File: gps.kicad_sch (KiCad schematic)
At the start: 7 parts, among them J3 50R SMA_Conn, U5 MAX-M10S

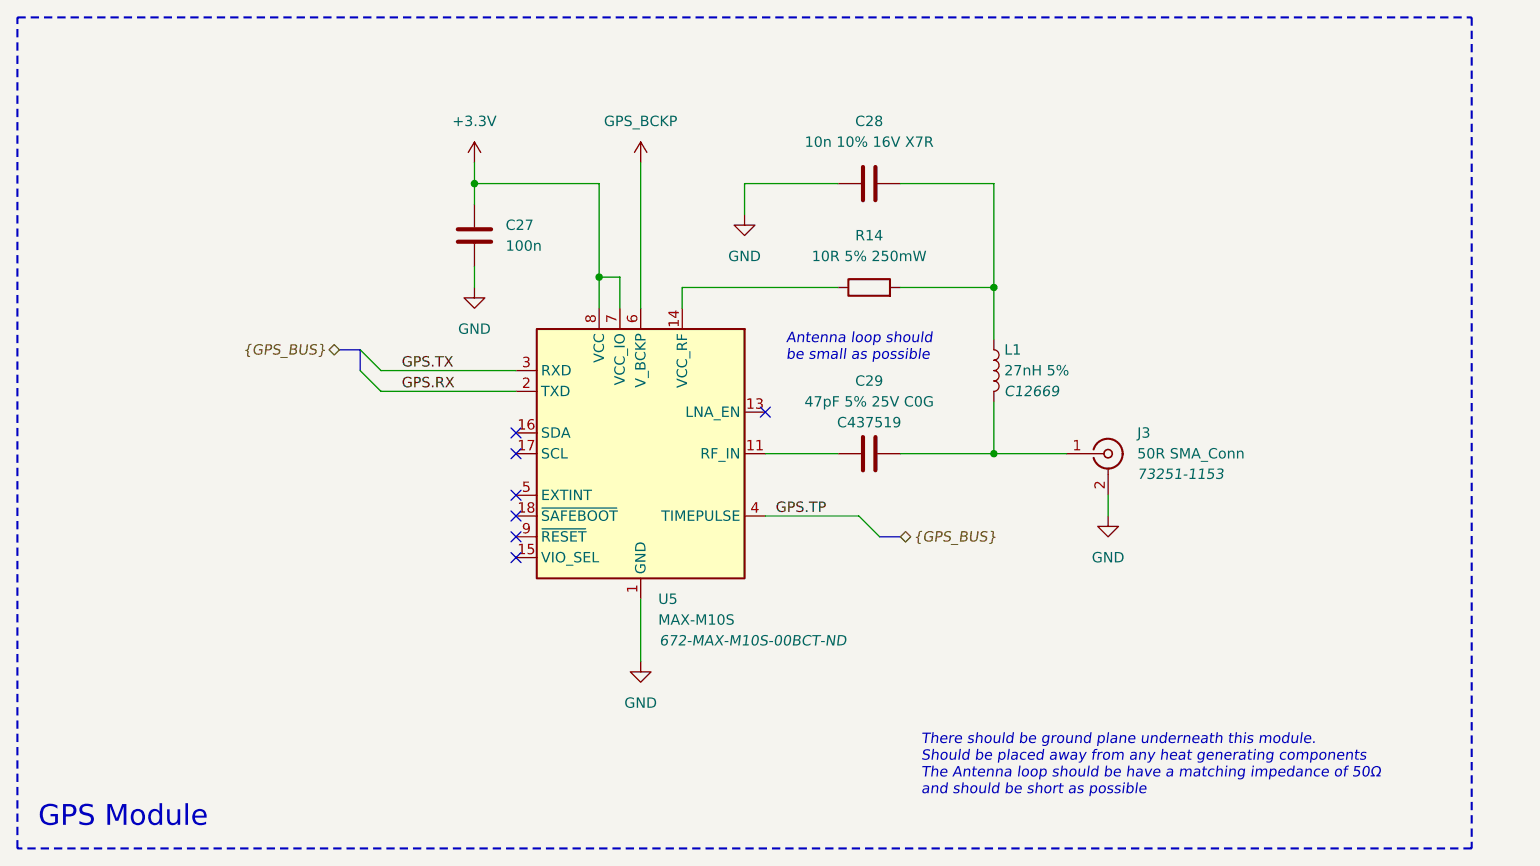
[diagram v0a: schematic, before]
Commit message: PCB Routing
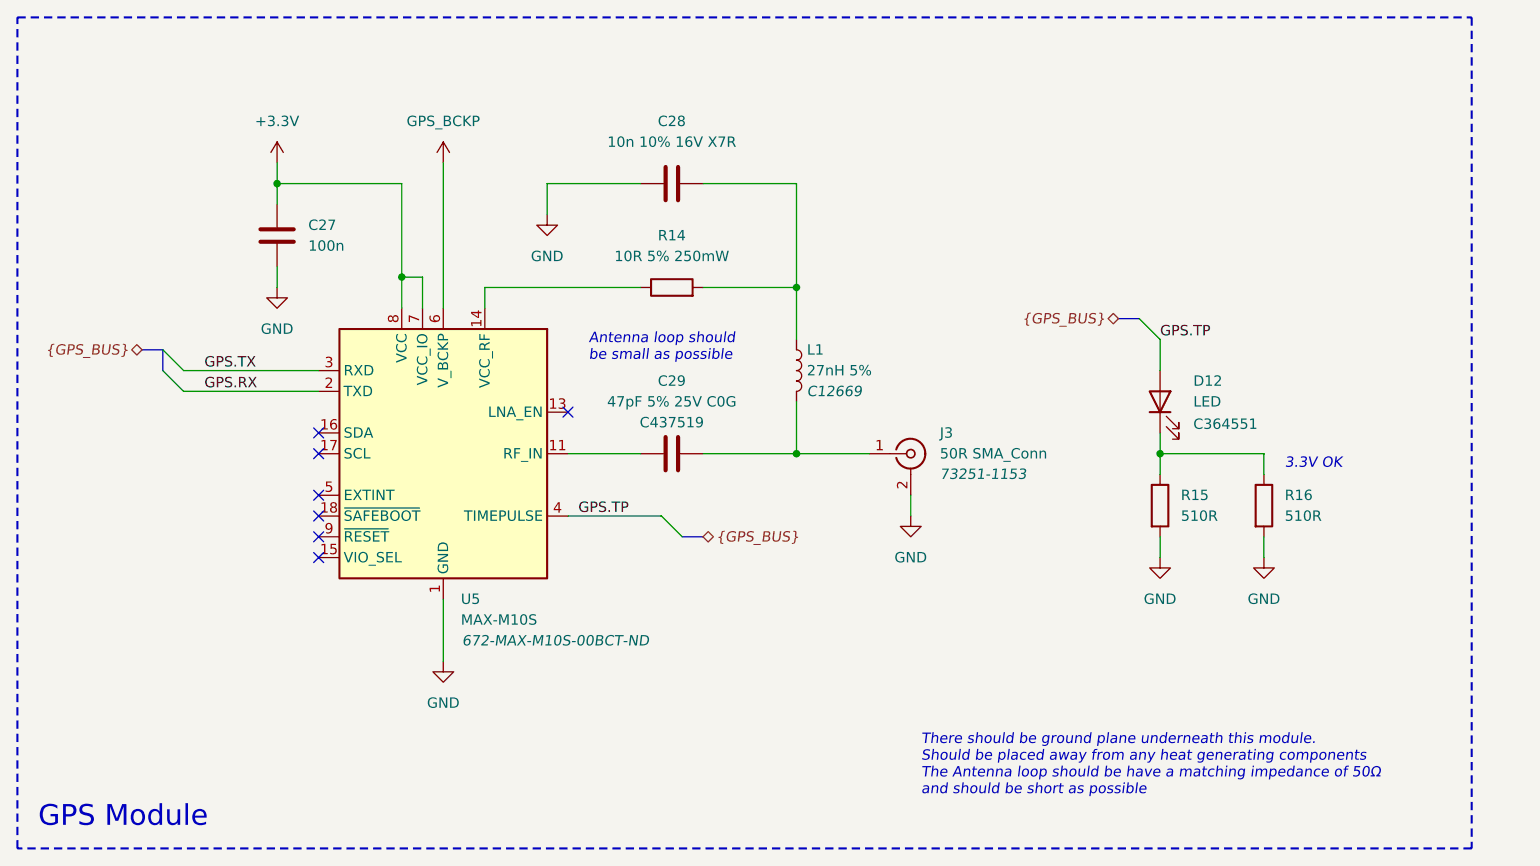
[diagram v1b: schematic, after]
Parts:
- added D12: LED, precision_clock:LED_LiteON_LTST-C281KGKT, symbol Device:LED
- added R15, R16: 510R, Resistor_SMD:R_0402_1005Metric, symbol Device:R
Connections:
- net GND: now also R15.2, R16.2
- net GPS.TP: now also D12.2 (A)
- new net: D12.1 (K), R15.1, R16.1
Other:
- note added: "3.3V OK"
- moved on the sheet: C27, C28, C29, J3, L1, R14, U5

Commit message: Major Changes
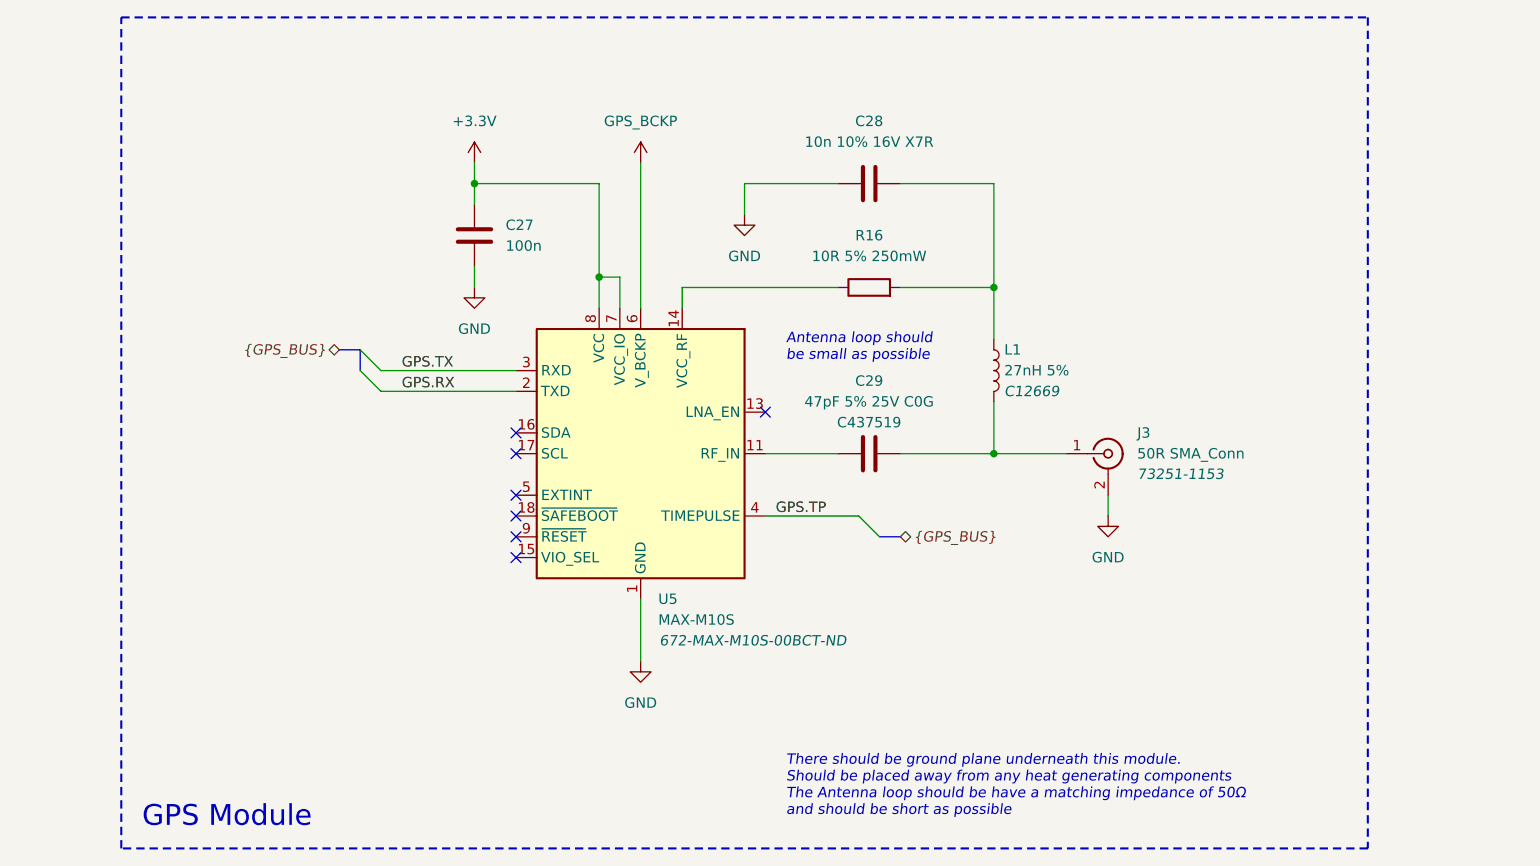
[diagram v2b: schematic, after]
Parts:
- removed D12: LED, precision_clock:LED_LiteON_LTST-C281KGKT, symbol Device:LED
- removed R15, R16: 510R, Resistor_SMD:R_0402_1005Metric, symbol Device:R
- renumbered R14 to R16
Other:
- note removed: "3.3V OK"
- moved on the sheet: C27, C28, C29, J3, L1, R16, U5
